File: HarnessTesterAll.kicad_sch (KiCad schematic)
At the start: 38 parts, among them J1 Input Tester, J2 Output Tester, J3 JTAG, SW1 Reset, U1 PIC32MX110F016D-IPT

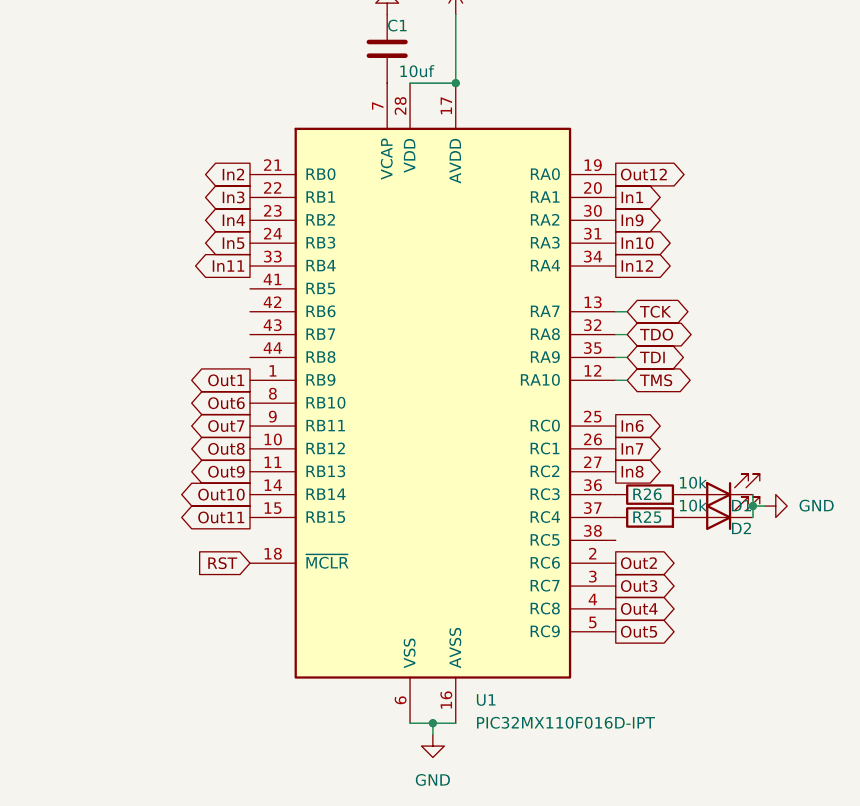
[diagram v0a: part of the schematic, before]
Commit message: Made a board laylout
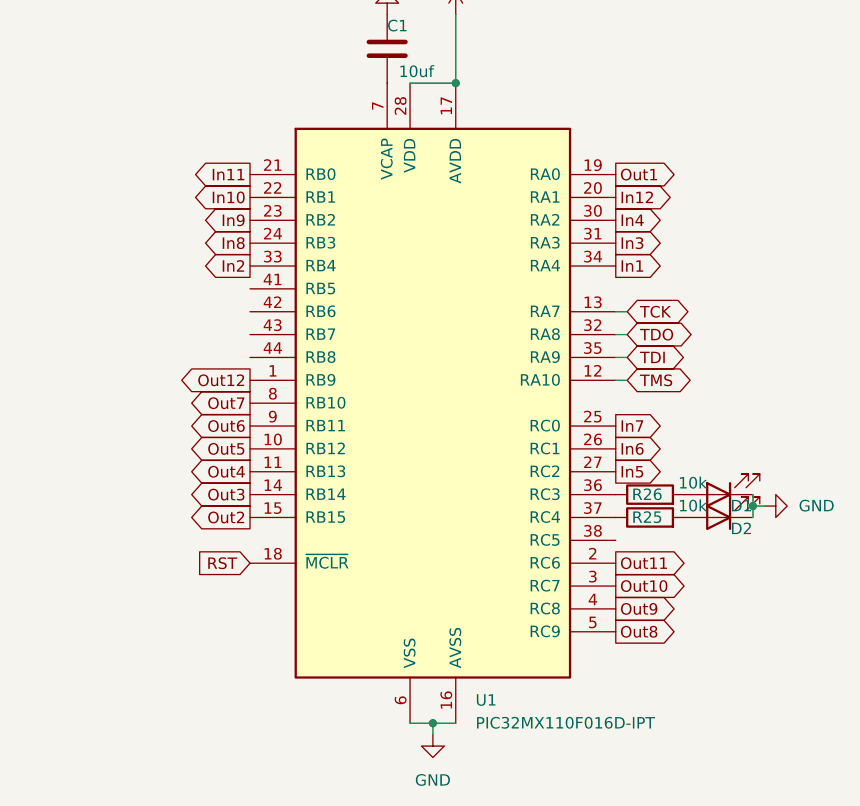
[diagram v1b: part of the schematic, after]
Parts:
- SW1: footprint (none) -> Button_Switch_SMD:SW_MEC_5GSH9
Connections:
- net In1: now also U1.34 (RA4); no longer U1.20 (RA1)
- net In10: now also U1.22 (RB1); no longer U1.31 (RA3)
- net In11: now also U1.21 (RB0); no longer U1.33 (RB4)
- net In12: now also U1.20 (RA1); no longer U1.34 (RA4)
- net In2: now also U1.33 (RB4); no longer U1.21 (RB0)
- net In3: now also U1.31 (RA3); no longer U1.22 (RB1)
- net In4: now also U1.30 (RA2); no longer U1.23 (RB2)
- net In5: now also U1.27 (RC2); no longer U1.24 (RB3)
- net In6: now also U1.26 (RC1); no longer U1.25 (RC0)
- net In7: now also U1.25 (RC0); no longer U1.26 (RC1)
- net In8: now also U1.24 (RB3); no longer U1.27 (RC2)
- net In9: now also U1.23 (RB2); no longer U1.30 (RA2)
- net Out1: now also U1.19 (RA0); no longer U1.1 (RB9)
- net Out10: now also U1.3 (RC7); no longer U1.14 (RB14)
- net Out11: now also U1.2 (RC6); no longer U1.15 (RB15)
- net Out12: now also U1.1 (RB9); no longer U1.19 (RA0)
- net Out2: now also U1.15 (RB15); no longer U1.2 (RC6)
- net Out3: now also U1.14 (RB14); no longer U1.3 (RC7)
- net Out4: now also U1.11 (RB13); no longer U1.4 (RC8)
- net Out5: now also U1.10 (RB12); no longer U1.5 (RC9)
- net Out6: now also U1.9 (RB11); no longer U1.8 (RB10)
- net Out7: now also U1.8 (RB10); no longer U1.9 (RB11)
- net Out8: now also U1.5 (RC9); no longer U1.10 (RB12)
- net Out9: now also U1.4 (RC8); no longer U1.11 (RB13)
